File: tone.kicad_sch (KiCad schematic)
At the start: 18 parts, among them Q6 2N3904, SW1 TONE

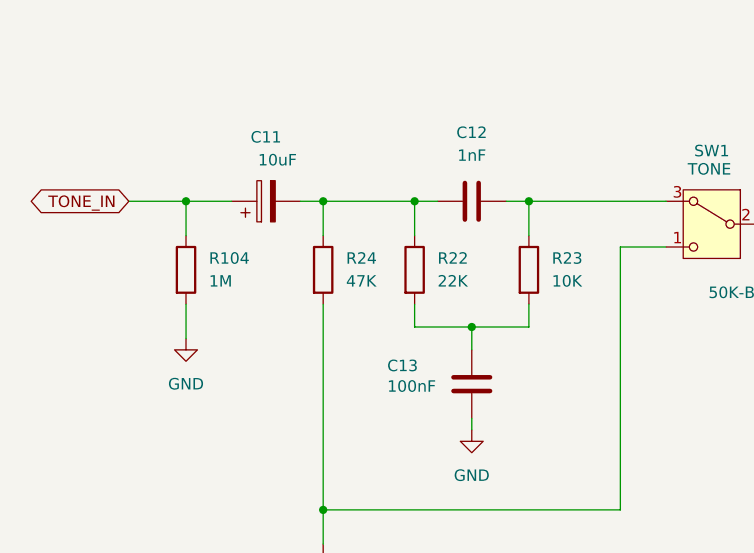
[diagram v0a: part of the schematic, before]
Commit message: Finalización de PCB (archivos fabricación pendientes)
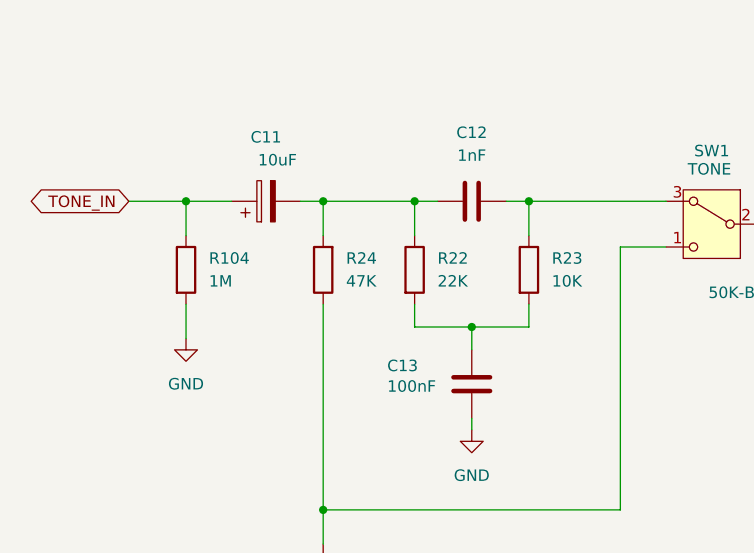
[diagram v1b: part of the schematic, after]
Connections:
- net at C11.2, C12.1, R22.1: now also R24.2; no longer R24.1
- net at R25.1, SW1.1 (C): now also R24.1; no longer R24.2
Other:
- moved on the sheet: R24
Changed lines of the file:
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@@
 	(symbol
 		(lib_id "Device:R")
-		(at 97.79 93.98 0)
+		(at 97.79 93.98 180)
 		(unit 1)
 		(exclude_from_sim no)
@@
 		(fields_autoplaced yes)
 		(property "Reference" "R24"
-			(at 100.33 92.71 0)
+			(at 100.33 92.7099 0)
 			(effects
 				(font
 					(size 1.27 1.27)
 				)
-				(justify left)
+				(justify right)
 			)
 		)
 		(property "Value" "47K"
-			(at 100.33 95.25 0)
+			(at 100.33 95.2499 0)
 			(effects
 				(font
 					(size 1.27 1.27)
 				)
-				(justify left)
+				(justify right)
 			)
 		)
 		(property "Footprint" "Resistor_THT:R_Axial_DIN0207_L6.3mm_D2.5mm_P7.62mm_Horizontal"
-			(at 96.012 93.98 90)
+			(at 99.568 93.98 90)
 			(effects
 				(font
